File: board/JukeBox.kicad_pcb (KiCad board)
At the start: 2 copper layers, 78.5 x 80 mm, 59 parts, among them J1 USB_C_Receptacle_USB2.0, J2 Conn_01x02, J3 Conn_01x04, J4 Conn_01x03, J5 Conn_01x08, SW1 SW_SPST, SW10 SW_SPST, SW11 SW_SPST, SW12 SW_SPST, SW2 SW_SPST, SW3 SW_SPST, SW4 SW_SPST, SW5 SW_SPST, SW6 SW_SPST, SW7 SW_SPST, SW8 SW_SPST, SW9 SW_SPST, U1 ATmega8U2-A, Y1 16MHz

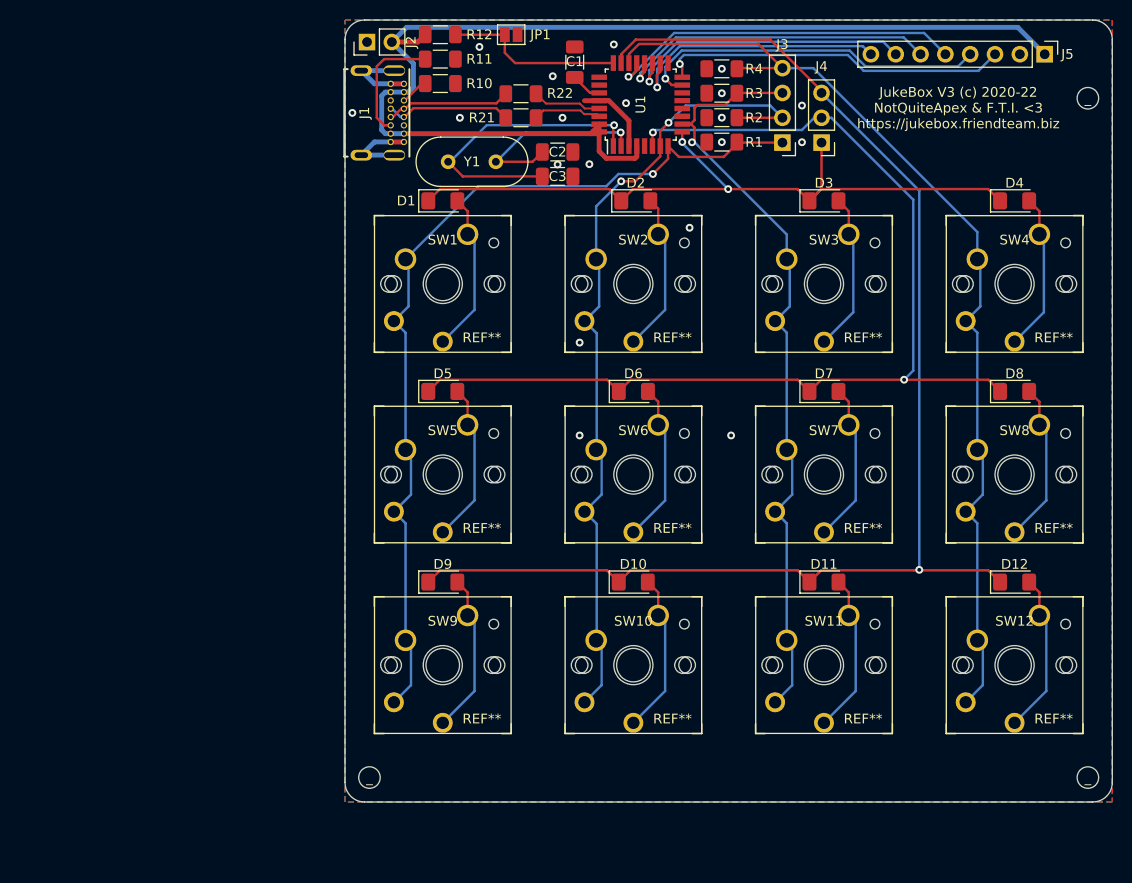
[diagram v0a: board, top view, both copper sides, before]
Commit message: import rp2040 minimal kicad project
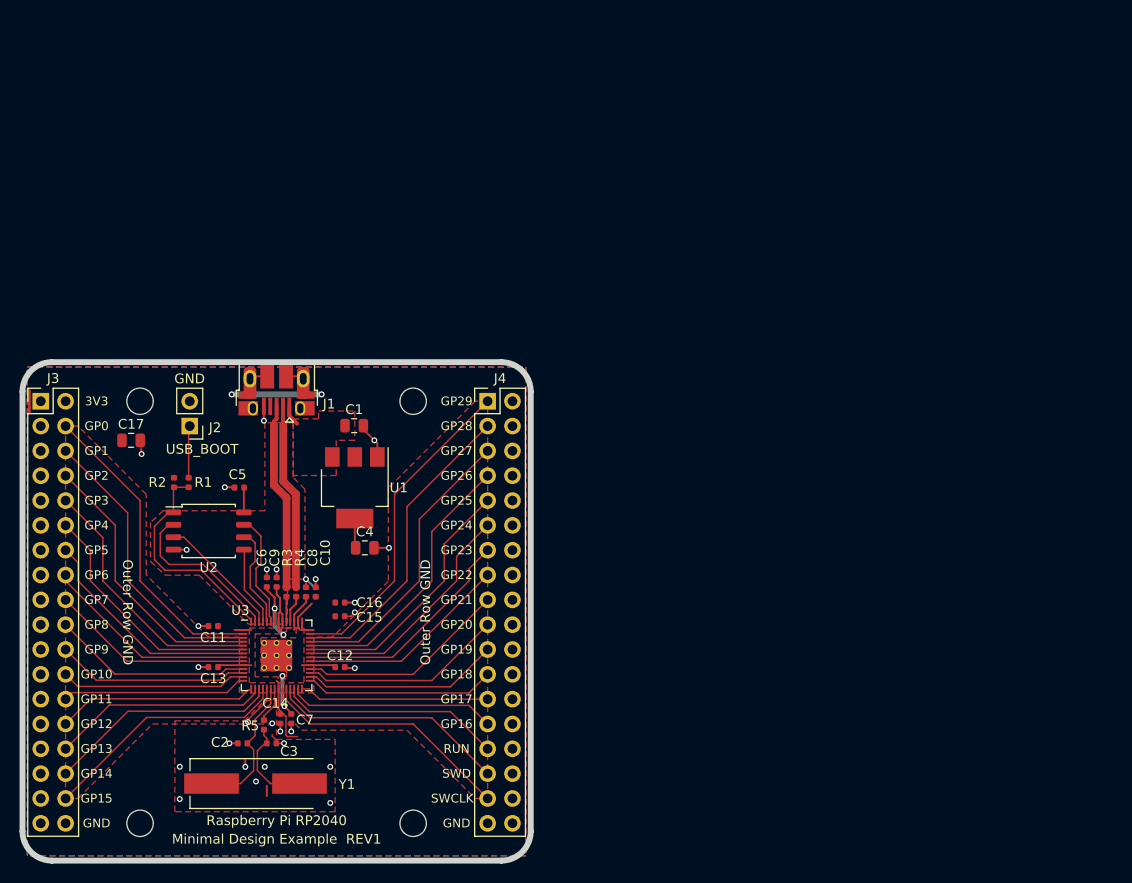
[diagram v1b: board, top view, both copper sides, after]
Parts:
- removed D1, D10, D11, D12, D2, D3, D4, D5, D6, D7, D8, D9: DIODE, Diode_SMD:D_1206_3216Metric_Pad1.42x1.75mm_HandSolder
- removed J5: Conn_01x08, Connector_PinHeader_2.54mm:PinHeader_1x08_P2.54mm_Vertical
- removed JP1: , Jumper:SolderJumper-2_P1.3mm_Open_Pad1.0x1.5mm
- removed R10, R11: 5.11k, Resistor_SMD:R_1206_3216Metric_Pad1.30x1.75mm_HandSolder
- removed R12: 10K, Resistor_SMD:R_1206_3216Metric_Pad1.30x1.75mm_HandSolder
- removed R21, R22: 22, Resistor_SMD:R_1206_3216Metric_Pad1.30x1.75mm_HandSolder
- removed REF** (x12): SW_Cherry_MX_1.00u_PCB, Button_Switch_Keyboard:SW_Cherry_MX_1.00u_PCB
- removed SW1, SW10, SW11, SW12, SW2, SW3, SW4, SW5, SW6, SW7, SW8, SW9: SW_SPST, jukebox-footprints:Kailh_PG1350
- removed _ (x3): MountingHole_2.2mm_M2, MountingHole:MountingHole_2.2mm_M2
- added C10: 1u, Capacitor_SMD:C_0402_1005Metric, F.Cu at (104.0, 93.5)
- added C11: 100n, Capacitor_SMD:C_0402_1005Metric, F.Cu at (93.5, 97.0)
- added C12: 100n, Capacitor_SMD:C_0402_1005Metric, F.Cu at (106.5, 101.2)
- added C13: 100n, Capacitor_SMD:C_0402_1005Metric, F.Cu at (93.5, 101.2)
- added C14: 100n, Capacitor_SMD:C_0402_1005Metric, F.Cu at (100.4, 106.5)
- added C15: 100n, Capacitor_SMD:C_0402_1005Metric, F.Cu at (106.5, 96.0)
- added C16: 100n, Capacitor_SMD:C_0402_1005Metric, F.Cu at (106.5, 94.6)
- added C17: 10u, Capacitor_SMD:C_0805_2012Metric, F.Cu at (85.1, 78.0)
- added C4: 10u, Capacitor_SMD:C_0805_2012Metric, F.Cu at (109.0, 89.0)
- added C5: 100n, Capacitor_SMD:C_0402_1005Metric, F.Cu at (96.2, 82.8)
- added C6: 100n, Capacitor_SMD:C_0402_1005Metric, F.Cu at (99.0, 92.5)
- added C7: 100n, Capacitor_SMD:C_0402_1005Metric, F.Cu at (101.5, 106.5)
- added C8: 1u, Capacitor_SMD:C_0402_1005Metric, F.Cu at (103.0, 93.5)
- added C9: 100n, Capacitor_SMD:C_0402_1005Metric, F.Cu at (100.0, 92.5)
- added H1: MountingHole, MountingHole:MountingHole_2.7mm_M2.5, F.Cu at (86.0, 74.0)
- added H2: MountingHole, MountingHole:MountingHole_2.7mm_M2.5, F.Cu at (114.0, 74.0)
- added H3: MountingHole, MountingHole:MountingHole_2.7mm_M2.5, F.Cu at (114.0, 117.2)
- added H4: MountingHole, MountingHole:MountingHole_2.7mm_M2.5, F.Cu at (86.0, 117.2)
- added R5: 1k, Capacitor_SMD:C_0402_1005Metric, F.Cu at (98.7, 107.1)
- added U2: W25Q128JVS, Package_SO:SOIC-8_5.23x5.23mm_P1.27mm, F.Cu at (93.0, 87.3)
- added U3: RP2040, RP2040_minimal:RP2040-QFN-56, F.Cu at (100.0, 100.0)
- C1: value 1uF -> 10u; footprint Capacitor_SMD:C_1206_3216Metric_Pad1.33x1.80mm_HandSolder -> Capacitor_SMD:C_0805_2012Metric
- C2, C3: value 18pF -> 27p; footprint Capacitor_SMD:C_1206_3216Metric_Pad1.33x1.80mm_HandSolder -> Capacitor_SMD:C_0402_1005Metric
- J1: value USB_C_Receptacle_USB2.0 -> USB_B_Micro; footprint jukebox-footprints:GCT_USB4085-GF-A_REVA4 -> RP2040_minimal:USB_Micro-B_Amphenol_10103594-0001LF_Horizontal_modified
- J3: value Conn_01x04 -> Conn_02x18_Odd_Even; footprint Connector_PinHeader_2.54mm:PinHeader_1x04_P2.54mm_Vertical -> Connector_PinHeader_2.54mm:PinHeader_2x18_P2.54mm_Vertical
- J4: value Conn_01x03 -> Conn_02x18_Odd_Even; footprint Connector_PinHeader_2.54mm:PinHeader_1x03_P2.54mm_Vertical -> Connector_PinHeader_2.54mm:PinHeader_2x18_P2.54mm_Vertical
- R1: value 10k -> 1k; footprint Resistor_SMD:R_1206_3216Metric_Pad1.30x1.75mm_HandSolder -> Capacitor_SMD:C_0402_1005Metric
- R2: value 10k -> DNF; footprint Resistor_SMD:R_1206_3216Metric_Pad1.30x1.75mm_HandSolder -> Capacitor_SMD:C_0402_1005Metric
- R3, R4: value 10k -> 27; footprint Resistor_SMD:R_1206_3216Metric_Pad1.30x1.75mm_HandSolder -> Capacitor_SMD:C_0402_1005Metric
- U1: value ATmega8U2-A -> NCP1117-3.3_SOT223; footprint Package_QFP:TQFP-32_7x7mm_P0.8mm -> Package_TO_SOT_SMD:SOT-223-3_TabPin2
- Y1: value 16MHz -> ABLS-12.000MHZ-B4-T; footprint Crystal:Crystal_HC49-4H_Vertical -> RP2040_minimal:Crystal_SMD_HC49-US
- moved J3 80.4 mm to (75.9, 74.0), turned to 0 degrees
- moved R4 69.0 mm to (102.0, 93.5), turned to -90 degrees
- moved C2 68.6 mm to (96.5, 109.0)
- moved R3 67.7 mm to (101.0, 93.5), turned to -90 degrees
- moved R2 67.3 mm to (89.5, 82.3), turned to -90 degrees
- moved Y1 66.6 mm to (97.8, 113.1)
- moved C3 65.0 mm to (99.5, 109.0), turned to 0 degrees
- moved R1 64.7 mm to (91.0, 82.3), turned to 90 degrees
- moved U1 48.9 mm to (108.0, 82.8), turned to -90 degrees
- moved C1 43.5 mm to (107.9, 76.5), turned to 0 degrees
- moved J2 43.3 mm to (91.1, 76.5), turned to 180 degrees
- moved J4 43.2 mm to (121.6, 74.0), turned to 0 degrees
- moved J1 28.7 mm to (100.0, 71.7), turned to 180 degrees
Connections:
- C1 pad 1: GND -> VBUS
- C1 pad 2: Net-(C1-Pad2) -> GND
- C2 pad 1: GND -> /XIN
- C2 pad 2: Net-(C2-Pad2) -> GND
- C3 pad 1: GND -> Net-(C3-Pad1)
- C3 pad 2: Net-(C3-Pad2) -> GND
- J2 pad 1: GND -> /~{USB_BOOT}
- J2 pad 2: +5V -> GND
- J3 pad 1: COL_1 -> GND
- J3 pad 2: COL_2 -> +3V3
- J3 pad 3: COL_3 -> GND
- J3 pad 4: COL_4 -> /GPIO0
- J4 pad 1: ROW_1 -> /GPIO29_ADC3
- J4 pad 2: ROW_2 -> GND
- J4 pad 3: ROW_3 -> /GPIO28_ADC2
- R1 pad 1: GND -> /QSPI_SS
- R1 pad 2: COL_1 -> /~{USB_BOOT}
- R2 pad 1: GND -> +3V3
- R2 pad 2: COL_2 -> /QSPI_SS
- R3 pad 1: GND -> /USB_D+
- R3 pad 2: COL_3 -> Net-(R3-Pad2)
- R4 pad 1: GND -> /USB_D-
- R4 pad 2: COL_4 -> Net-(R4-Pad2)
- U1 pad 1: Net-(C3-Pad2) -> GND
- U1 pad 2: Net-(C2-Pad2) -> +3V3
- U1 pad 3: GND -> VBUS
- Y1 pad 1: Net-(C3-Pad2) -> /XIN
- Y1 pad 2: Net-(C2-Pad2) -> Net-(C3-Pad1)
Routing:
- net ROW_3: track 138.8 -> 0.00 mm, vias 1 -> 0
- net +5V: track 117.2 -> 0.00 mm
- net ROW_2: track 112.4 -> 0.00 mm, vias 2 -> 0
- net COL_4: track 101.4 -> 0.00 mm
- net COL_1: track 94.3 -> 0.00 mm, vias 1 -> 0
- net COL_2: track 84.4 -> 0.00 mm, vias 2 -> 0
- net COL_3: track 80.4 -> 0.00 mm, vias 1 -> 0
- net ROW_1: track 75.8 -> 0.00 mm, vias 2 -> 0
- net +3V3: track 0.00 -> 45.2 mm, vias 0 -> 2
- net CS: track 37.0 -> 0.00 mm, vias 1 -> 0
- net CLK: track 36.3 -> 0.00 mm, vias 1 -> 0
- net DIN: track 35.8 -> 0.00 mm, vias 1 -> 0
- net DC: track 33.2 -> 0.00 mm, vias 1 -> 0
- net /GPIO29_ADC3: track 0.00 -> 33.2 mm
- net /GPIO0: track 0.00 -> 31.8 mm
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- added copper zone on F.Cu, net +1V1
- added copper zone on F.Cu, net +3V3
- added copper zone on F.Cu, net VBUS
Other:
- board size 78.5 x 80 mm -> 52 x 51 mm
- rule pad_to_mask_clearance: 0 -> 0.051
- board text added: "3V3"
- board text added: "GND"
- board text added: "GP0"
- board text added: "GP1"
- board text added: "GP10"
- board text added: "GP11"
- board text added: "GP12"
- board text added: "GP13"
- board text added: "GP14"
- board text added: "GP15"
- board text added: "GP16"
- board text added: "GP17"
- board text added: "GP18"
- board text added: "GP19"
- board text added: "GP2"
- board text added: "GP20"
- board text added: "GP21"
- board text added: "GP22"
- board text added: "GP23"
- board text added: "GP24"
- board text added: "GP25"
- board text added: "GP26"
- board text added: "GP27"
- board text added: "GP28"
- board text added: "GP29"
- board text added: "GP3"
- board text added: "GP4"
- board text added: "GP5"
- board text added: "GP6"
- board text added: "GP7"
- board text added: "GP8"
- board text added: "GP9"
- board text added: "Minimal Design Example REV1"
- board text added: "Outer Row GND"
- board text added: "RUN"
- board text added: "Raspberry Pi RP2040"
- board text added: "SWCLK"
- board text added: "SWD"
- board text added: "USB_BOOT"
- board text removed: "JukeBox V3 (c) 2020-22 NotQuiteApex & F.T.I. <3 https://jukebox.friendteam.biz"

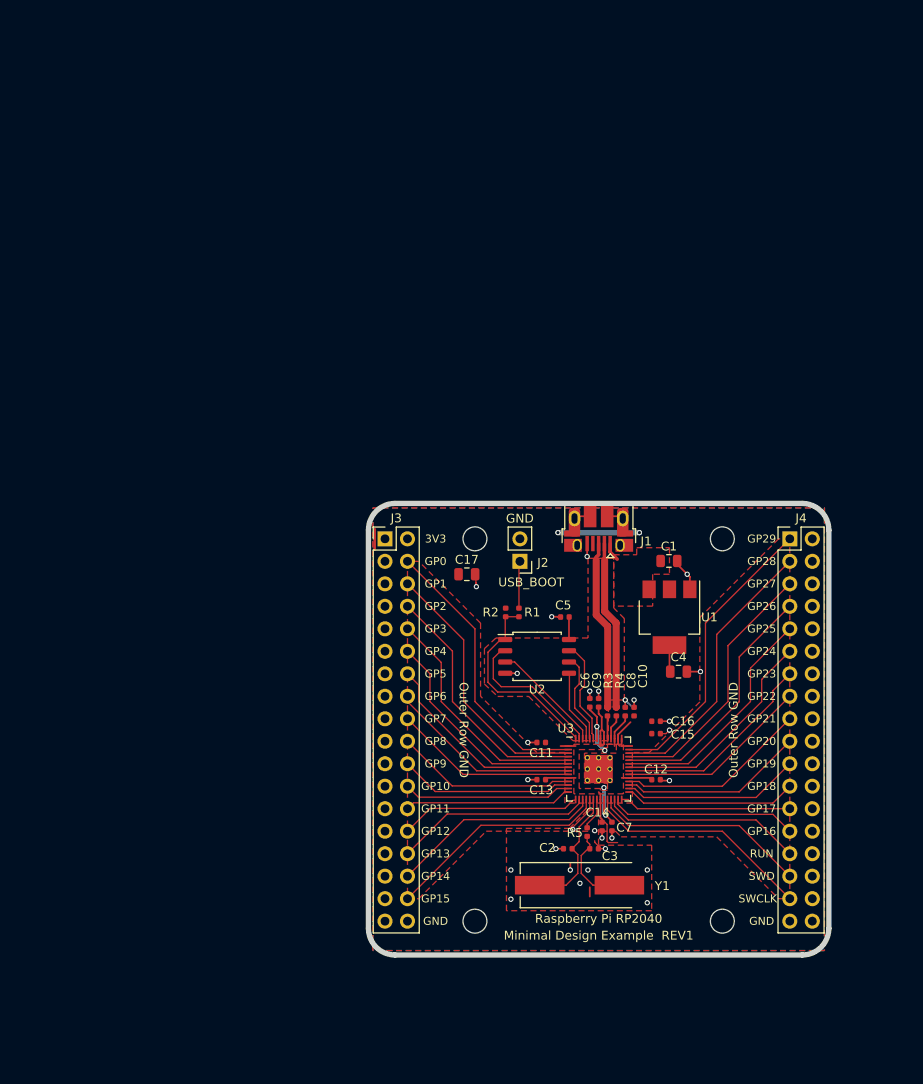
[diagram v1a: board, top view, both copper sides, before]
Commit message: first pass over pcb
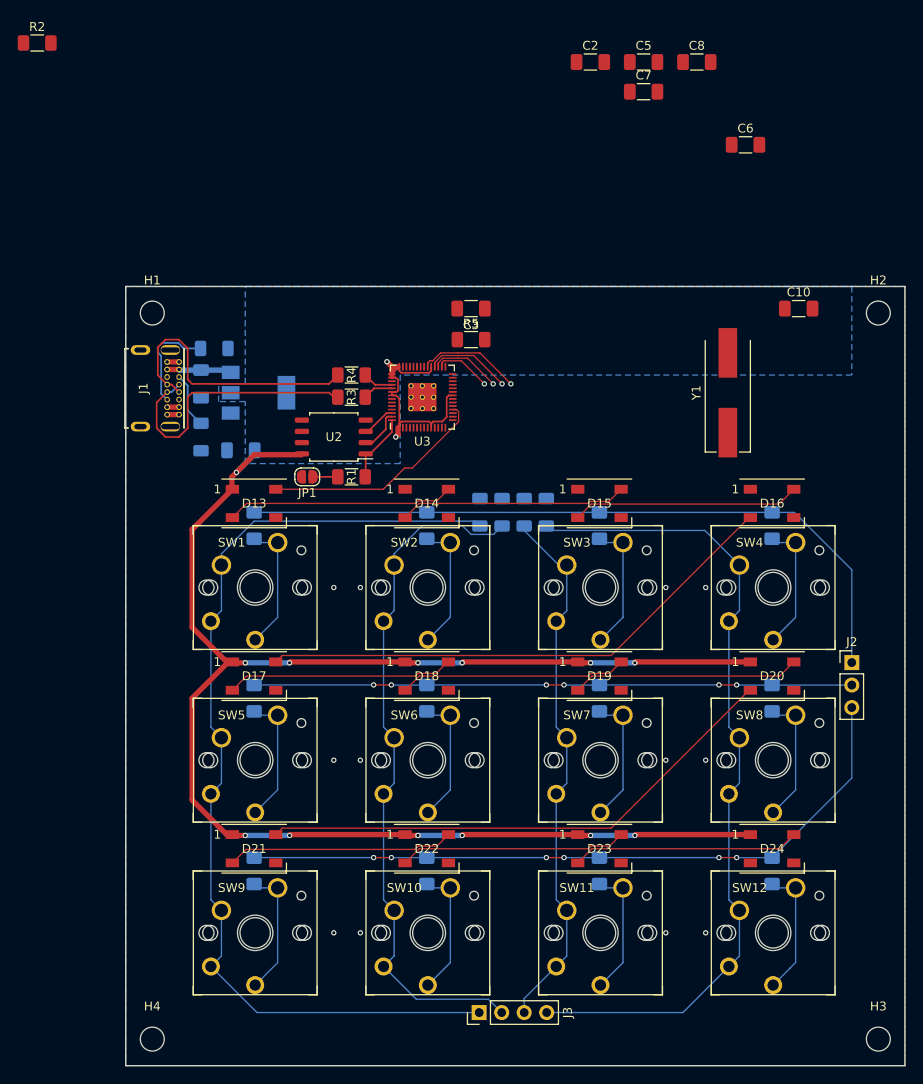
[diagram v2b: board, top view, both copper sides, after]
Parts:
- removed C11, C12, C13, C14, C15, C16, C9: 100n, Capacitor_SMD:C_0402_1005Metric
- removed C17: 10u, Capacitor_SMD:C_0805_2012Metric
- removed J4: Conn_02x18_Odd_Even, Connector_PinHeader_2.54mm:PinHeader_2x18_P2.54mm_Vertical
- added D1: DIODE, Diode_SMD:D_1206_3216Metric_Pad1.42x1.75mm_HandSolder, B.Cu at (61.1, 72.5)
- added D10: DIODE, Diode_SMD:D_1206_3216Metric_Pad1.42x1.75mm_HandSolder, B.Cu at (80.6, 111.5)
- added D11: DIODE, Diode_SMD:D_1206_3216Metric_Pad1.42x1.75mm_HandSolder, B.Cu at (100.1, 111.5)
- added D12: DIODE, Diode_SMD:D_1206_3216Metric_Pad1.42x1.75mm_HandSolder, B.Cu at (119.6, 111.5)
- added D13: WS2812B, LED_SMD:LED_WS2812B_PLCC4_5.0x5.0mm_P3.2mm, F.Cu at (61.1, 70.0)
- added D14: WS2812B, LED_SMD:LED_WS2812B_PLCC4_5.0x5.0mm_P3.2mm, F.Cu at (80.6, 70.0)
- added D15: WS2812B, LED_SMD:LED_WS2812B_PLCC4_5.0x5.0mm_P3.2mm, F.Cu at (100.1, 70.0)
- added D16: WS2812B, LED_SMD:LED_WS2812B_PLCC4_5.0x5.0mm_P3.2mm, F.Cu at (119.6, 70.0)
- added D17: WS2812B, LED_SMD:LED_WS2812B_PLCC4_5.0x5.0mm_P3.2mm, F.Cu at (61.1, 89.5)
- added D18: WS2812B, LED_SMD:LED_WS2812B_PLCC4_5.0x5.0mm_P3.2mm, F.Cu at (80.6, 89.5)
- added D19: WS2812B, LED_SMD:LED_WS2812B_PLCC4_5.0x5.0mm_P3.2mm, F.Cu at (100.1, 89.5)
- added D2: DIODE, Diode_SMD:D_1206_3216Metric_Pad1.42x1.75mm_HandSolder, B.Cu at (80.6, 72.5)
- added D20: WS2812B, LED_SMD:LED_WS2812B_PLCC4_5.0x5.0mm_P3.2mm, F.Cu at (119.6, 89.5)
- added D21: WS2812B, LED_SMD:LED_WS2812B_PLCC4_5.0x5.0mm_P3.2mm, F.Cu at (61.1, 109.0)
- added D22: WS2812B, LED_SMD:LED_WS2812B_PLCC4_5.0x5.0mm_P3.2mm, F.Cu at (80.6, 109.0)
- added D23: WS2812B, LED_SMD:LED_WS2812B_PLCC4_5.0x5.0mm_P3.2mm, F.Cu at (100.1, 109.0)
- added D24: WS2812B, LED_SMD:LED_WS2812B_PLCC4_5.0x5.0mm_P3.2mm, F.Cu at (119.6, 109.0)
- added D3: DIODE, Diode_SMD:D_1206_3216Metric_Pad1.42x1.75mm_HandSolder, B.Cu at (100.1, 72.5)
- added D4: DIODE, Diode_SMD:D_1206_3216Metric_Pad1.42x1.75mm_HandSolder, B.Cu at (119.6, 72.5)
- added D5: DIODE, Diode_SMD:D_1206_3216Metric_Pad1.42x1.75mm_HandSolder, B.Cu at (61.1, 92.0)
- added D6: DIODE, Diode_SMD:D_1206_3216Metric_Pad1.42x1.75mm_HandSolder, B.Cu at (80.6, 92.0)
- added D7: DIODE, Diode_SMD:D_1206_3216Metric_Pad1.42x1.75mm_HandSolder, B.Cu at (100.1, 92.0)
- added D8: DIODE, Diode_SMD:D_1206_3216Metric_Pad1.42x1.75mm_HandSolder, B.Cu at (119.6, 92.0)
- added D9: DIODE, Diode_SMD:D_1206_3216Metric_Pad1.42x1.75mm_HandSolder, B.Cu at (61.1, 111.5)
- added JP1: SolderJumper_2_Open, Jumper:SolderJumper-2_P1.3mm_Open_RoundedPad1.0x1.5mm, F.Cu at (67.1, 67.0)
- added R11: 10k, Resistor_SMD:R_1206_3216Metric_Pad1.30x1.75mm_HandSolder, B.Cu at (86.6, 71.0)
- added R12: 10k, Resistor_SMD:R_1206_3216Metric_Pad1.30x1.75mm_HandSolder, B.Cu at (89.1, 71.0)
- added R13: 10k, Resistor_SMD:R_1206_3216Metric_Pad1.30x1.75mm_HandSolder, B.Cu at (91.6, 71.0)
- added R14: 10k, Resistor_SMD:R_1206_3216Metric_Pad1.30x1.75mm_HandSolder, B.Cu at (94.1, 71.0)
- added R6: 5.11k, Resistor_SMD:R_1206_3216Metric_Pad1.30x1.75mm_HandSolder, B.Cu at (55.1, 62.5)
- added R7: 5.11k, Resistor_SMD:R_1206_3216Metric_Pad1.30x1.75mm_HandSolder, B.Cu at (56.6, 52.5)
- added SW1: SW_SPST, RP2040_minimal:Kailh_Choc_MX_Key, F.Cu at (61.1, 79.5)
- added SW10: SW_SPST, RP2040_minimal:Kailh_Choc_MX_Key, F.Cu at (80.6, 118.5)
- added SW11: SW_SPST, RP2040_minimal:Kailh_Choc_MX_Key, F.Cu at (100.1, 118.5)
- added SW12: SW_SPST, RP2040_minimal:Kailh_Choc_MX_Key, F.Cu at (119.6, 118.5)
- added SW2: SW_SPST, RP2040_minimal:Kailh_Choc_MX_Key, F.Cu at (80.6, 79.5)
- added SW3: SW_SPST, RP2040_minimal:Kailh_Choc_MX_Key, F.Cu at (100.1, 79.5)
- added SW4: SW_SPST, RP2040_minimal:Kailh_Choc_MX_Key, F.Cu at (119.6, 79.5)
- added SW5: SW_SPST, RP2040_minimal:Kailh_Choc_MX_Key, F.Cu at (61.1, 99.0)
- added SW6: SW_SPST, RP2040_minimal:Kailh_Choc_MX_Key, F.Cu at (80.6, 99.0)
- added SW7: SW_SPST, RP2040_minimal:Kailh_Choc_MX_Key, F.Cu at (100.1, 99.0)
- added SW8: SW_SPST, RP2040_minimal:Kailh_Choc_MX_Key, F.Cu at (119.6, 99.0)
- added SW9: SW_SPST, RP2040_minimal:Kailh_Choc_MX_Key, F.Cu at (61.1, 118.5)
- C1, C4: footprint Capacitor_SMD:C_0805_2012Metric -> Capacitor_SMD:C_1206_3216Metric_Pad1.33x1.80mm_HandSolder; moved to B.Cu
- C10, C2, C3, C5, C6, C7, C8: footprint Capacitor_SMD:C_0402_1005Metric -> Capacitor_SMD:C_1206_3216Metric_Pad1.33x1.80mm_HandSolder
- J1: value USB_B_Micro -> USB_C_Receptacle_USB2.0; footprint RP2040_minimal:USB_Micro-B_Amphenol_10103594-0001LF_Horizontal_modified -> RP2040_minimal:GCT_USB4085-GF-A_REVA4
- J2: value Conn_01x02 -> Conn_01x03; footprint Connector_PinHeader_2.54mm:PinHeader_1x02_P2.54mm_Vertical -> Connector_PinHeader_2.54mm:PinHeader_1x03_P2.54mm_Vertical
- J3: value Conn_02x18_Odd_Even -> Conn_01x04; footprint Connector_PinHeader_2.54mm:PinHeader_2x18_P2.54mm_Vertical -> Connector_PinHeader_2.54mm:PinHeader_1x04_P2.54mm_Vertical
- R1, R2, R3, R4, R5: footprint Capacitor_SMD:C_0402_1005Metric -> Resistor_SMD:R_1206_3216Metric_Pad1.30x1.75mm_HandSolder
- U1: moved to B.Cu
- moved C2 88.9 mm to (99.1, 20.1), turned to 0 degrees
- moved R2 83.3 mm to (36.6, 18.0), turned to 0 degrees
- moved C7 83.1 mm to (105.1, 23.5), turned to 0 degrees
- moved C8 73.8 mm to (111.1, 20.1), turned to 0 degrees
- moved C6 65.4 mm to (116.6, 29.5), turned to 0 degrees
- moved C5 63.3 mm to (105.1, 20.1), turned to 0 degrees
- moved C3 62.6 mm to (85.6, 48.0), turned to 180 degrees
- moved Y1 58.1 mm to (114.6, 57.5), turned to 90 degrees
- moved R5 57.1 mm to (85.6, 51.5), turned to 0 degrees
- moved C1 56.5 mm to (55.1, 56.5), turned to -90 degrees
- moved C4 55.4 mm to (59.6, 64.0), turned to 180 degrees
- moved J3 54.5 mm to (86.5, 127.5), turned to 90 degrees
- moved J1 53.5 mm to (48.6, 57.0), turned to -90 degrees
- moved U1 52.9 mm to (61.6, 57.5), turned to 0 degrees
- moved C10 49.2 mm to (122.6, 48.0), turned to 0 degrees
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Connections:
- J2 pad 1: /~{USB_BOOT} -> /GPIO16
- J2 pad 2: GND -> /GPIO17
- J3 pad 1: GND -> /GPIO19
- J3 pad 2: +3V3 -> /GPIO20
- J3 pad 3: GND -> /GPIO21
- J3 pad 4: /GPIO0 -> /GPIO22
- R1 pad 1: /QSPI_SS -> /~{USB_BOOT}
- R1 pad 2: /~{USB_BOOT} -> /QSPI_SS
- U3 pad 2: /GPIO0 -> /DBGRX
- U3 pad 24: /SWCLK -> /DBGSC
- U3 pad 25: /SWD -> /DBGSD
- U3 pad 3: /GPIO1 -> /DBGTX
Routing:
- net +3V3: track 45.2 -> 206.0 mm, vias 2 -> 15
- net /GPIO19: track 20.1 -> 118.9 mm, vias 0 -> 1
- net /GPIO22: track 21.8 -> 105.9 mm, vias 0 -> 1
- net /GPIO20: track 20.8 -> 87.0 mm, vias 0 -> 1
- net Net-(D16-Pad2): track 0.00 -> 60.4 mm
- net Net-(D20-Pad2): track 0.00 -> 60.4 mm
- net /GPIO18: track 19.5 -> 79.2 mm, vias 0 -> 6
- net /GPIO16: track 21.2 -> 80.7 mm
- net /GPIO21: track 21.5 -> 71.2 mm, vias 0 -> 1
- net /GPIO17: track 19.4 -> 67.5 mm, vias 0 -> 6
- net /GPIO29_ADC3: track 33.2 -> 0.00 mm
- net GND: track 34.8 -> 2.70 mm, vias 28 -> 12
- net /GPIO0: track 31.8 -> 0.00 mm
- net /GPIO28_ADC2: track 31.6 -> 0.00 mm
- net /GPIO1: track 30.2 -> 0.00 mm
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- added copper zone on B.Cu, net +3V3
- removed copper zone on F.Cu, net +1V1
- removed copper zone on F.Cu, net +3V3
- removed copper zone on F.Cu, net VBUS
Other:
- board size 52 x 51 mm -> 88 x 88 mm
- board text removed: "3V3"
- board text removed: "GND"
- board text removed: "GP0"
- board text removed: "GP1"
- board text removed: "GP10"
- board text removed: "GP11"
- board text removed: "GP12"
- board text removed: "GP13"
- board text removed: "GP14"
- board text removed: "GP15"
- board text removed: "GP16"
- board text removed: "GP17"
- board text removed: "GP18"
- board text removed: "GP19"
- board text removed: "GP2"
- board text removed: "GP20"
- board text removed: "GP21"
- board text removed: "GP22"
- board text removed: "GP23"
- board text removed: "GP24"
- board text removed: "GP25"
- board text removed: "GP26"
- board text removed: "GP27"
- board text removed: "GP28"
- board text removed: "GP29"
- board text removed: "GP3"
- board text removed: "GP4"
- board text removed: "GP5"
- board text removed: "GP6"
- board text removed: "GP7"
- board text removed: "GP8"
- board text removed: "GP9"
- board text removed: "Minimal Design Example REV1"
- board text removed: "Outer Row GND"
- board text removed: "RUN"
- board text removed: "Raspberry Pi RP2040"
- board text removed: "SWCLK"
- board text removed: "SWD"
- board text removed: "USB_BOOT"
